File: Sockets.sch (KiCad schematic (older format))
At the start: 55 parts, among them J10 CA58SUB-B, J11 PC6 EPSON MAINBOARD, J12 Y AXIS, J13 Z AXIS, J14 LED 1, J15 LED 2, J6 LIMIT Y BACK, J7 LIMIT Y FRONT, J8 LIMIT Z UP, J9 LIMIT Z DOWN, Q1 2N7002K, Q2 2N7002K, Q3 2N7002K, Q4 2N7002K, Q5 2N7002K, Q6 2N7002K, Q7 2N7002K, U5 74HC245

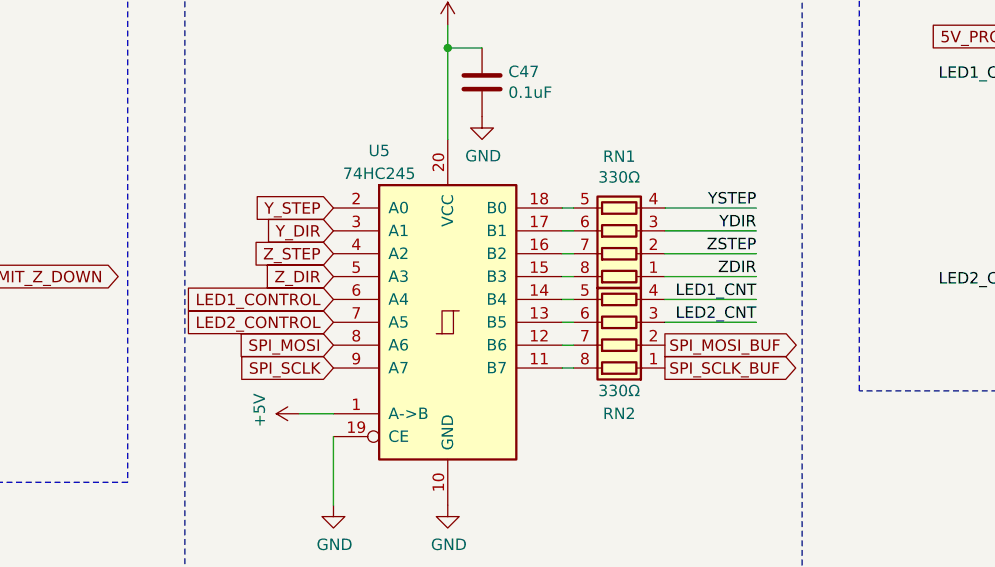
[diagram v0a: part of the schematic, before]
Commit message: Routing almost finished
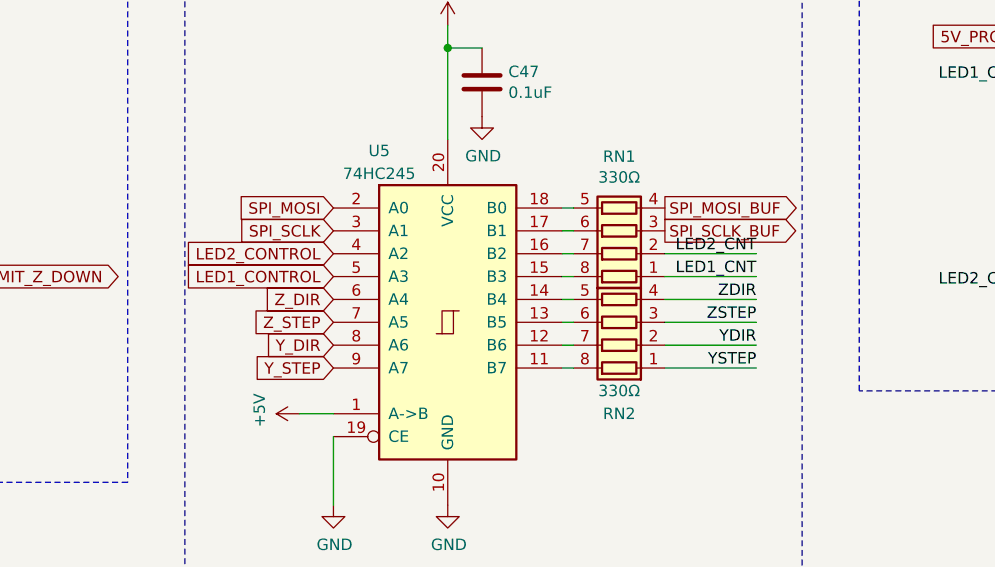
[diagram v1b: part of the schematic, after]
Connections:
- net LED1_CNT: now also RN1.1 (R1.1); no longer RN2.4 (R4.1)
- net LED1_CONTROL: now also U5.5 (A3); no longer U5.6 (A4)
- net LED2_CNT: now also RN1.2 (R2.1); no longer RN2.3 (R3.1)
- net LED2_CONTROL: now also U5.4 (A2); no longer U5.7 (A5)
- net SPI_MOSI: now also U5.2 (A0); no longer U5.8 (A6)
- net SPI_MOSI_BUF: now also RN1.4 (R4.1); no longer RN2.2 (R2.1)
- net SPI_SCLK: now also U5.3 (A1); no longer U5.9 (A7)
- net SPI_SCLK_BUF: now also RN1.3 (R3.1); no longer RN2.1 (R1.1)
- net YDIR: now also RN2.2 (R2.1); no longer RN1.3 (R3.1)
- net YSTEP: now also RN2.1 (R1.1); no longer RN1.4 (R4.1)
- net Y_DIR: now also U5.8 (A6); no longer U5.3 (A1)
- net Y_STEP: now also U5.9 (A7); no longer U5.2 (A0)
- net ZDIR: now also RN2.4 (R4.1); no longer RN1.1 (R1.1)
- net ZSTEP: now also RN2.3 (R3.1); no longer RN1.2 (R2.1)
- net Z_DIR: now also U5.6 (A4); no longer U5.5 (A3)
- net Z_STEP: now also U5.7 (A5); no longer U5.4 (A2)
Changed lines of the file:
@@
 Text Notes 4550 2600 0    50   ~ 0
 PE Signal Output to Emulate PE Sensor
-Text GLabel 4700 5600 0    50   Input ~ 0
+Text GLabel 4700 6300 0    50   Input ~ 0
 Y_STEP
-Text GLabel 4700 5700 0    50   Input ~ 0
+Text GLabel 4700 6200 0    50   Input ~ 0
 Y_DIR
+Text GLabel 4700 6100 0    50   Input ~ 0
+Z_STEP
+Text GLabel 4700 6000 0    50   Input ~ 0
+Z_DIR
+Text GLabel 4700 5900 0    50   Input ~ 0
+LED1_CONTROL
 Text GLabel 4700 5800 0    50   Input ~ 0
-Z_STEP
-Text GLabel 4700 5900 0    50   Input ~ 0
-Z_DIR
-Text GLabel 4700 6000 0    50   Input ~ 0
-LED1_CONTROL
-Text GLabel 4700 6100 0    50   Input ~ 0
 LED2_CONTROL
 $Comp
@@
 Wire Wire Line
 	4550 6500 4700 6500
-Text Label 6550 5600 2    50   ~ 0
+Text Label 6550 6300 2    50   ~ 0
 YSTEP
-Text Label 6550 5700 2    50   ~ 0
+Text Label 6550 6200 2    50   ~ 0
 YDIR
+Text Label 6550 6100 2    50   ~ 0
+ZSTEP
+Text Label 6550 6000 2    50   ~ 0
+ZDIR
+Text Label 6550 5900 2    50   ~ 0
+LED1_CNT
 Text Label 6550 5800 2    50   ~ 0
-ZSTEP
-Text Label 6550 5900 2    50   ~ 0
-ZDIR
-Text Label 6550 6000 2    50   ~ 0
-LED1_CNT
-Text Label 6550 6100 2    50   ~ 0
 LED2_CNT
 Text Label 7700 5050 2    50   ~ 0
@@
 	5700 6300 5750 6300
 Wire Wire Line
-	6150 5600 6550 5600
+	6150 6300 6550 6300
 Wire Wire Line
-	6150 5700 6550 5700
+	6150 6200 6550 6200
+Wire Wire Line
+	6150 6100 6550 6100
+Wire Wire Line
+	6150 6000 6550 6000
 Wire Wire Line
 	6150 5800 6550 5800
 Wire Wire Line
 	6150 5900 6550 5900
-Wire Wire Line
-	6150 6000 6550 6000
-Wire Wire Line
-	6150 6100 6550 6100
 Wire Notes Line
 	4050 4450 6750 4450
@@
 Text Notes 7500 2650 0    50   ~ 0
 Optional Step/DIR Outputs
-Text GLabel 4700 6300 0    50   Input ~ 0
+Text GLabel 4700 5700 0    50   Input ~ 0
 SPI_SCLK
-Text GLabel 4700 6200 0    50   Input ~ 0
+Text GLabel 4700 5600 0    50   Input ~ 0
 SPI_MOSI
-Text GLabel 6150 6200 2    50   Output ~ 0
+Text GLabel 6150 5600 2    50   Output ~ 0
 SPI_MOSI_BUF
-Text GLabel 6150 6300 2    50   Output ~ 0
+Text GLabel 6150 5700 2    50   Output ~ 0
 SPI_SCLK_BUF
 Wire Wire Line
